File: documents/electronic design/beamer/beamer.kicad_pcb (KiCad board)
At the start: 2 copper layers, 23 parts, among them P1 CONN_01X20, P2 CONN_01X20, T1 2N7002K, T10 2N7002K, T2 2N7002K, T3 2N7002K, T4 2N7002K, T5 2N7002K, T6 2N7002K, T7 2N7002K, T8 2N7002K, T9 2N7002K, U1 NRF24L01-BRKOUT

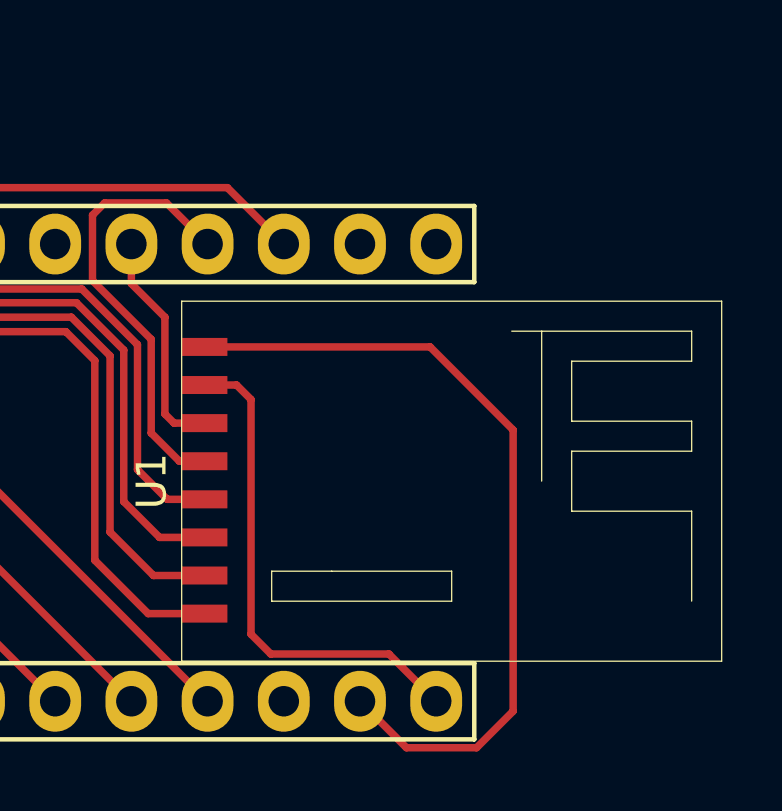
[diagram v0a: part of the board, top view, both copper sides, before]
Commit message: add capacitor to pcb
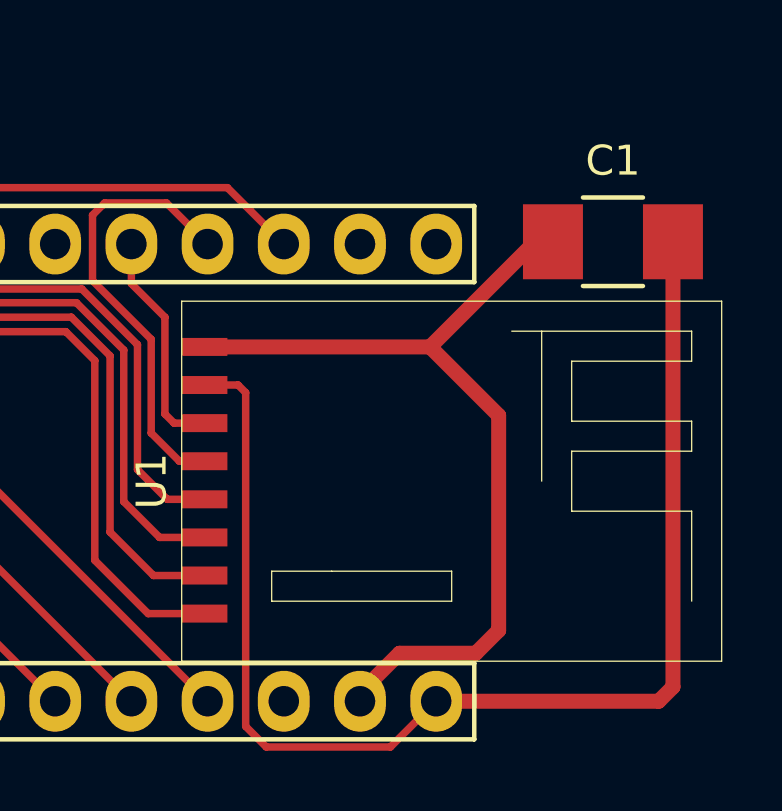
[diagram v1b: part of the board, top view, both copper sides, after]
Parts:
- added C1: C, Capacitors_SMD:C_1210_HandSoldering, F.Cu at (237.5, 44.2)
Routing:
- net +3V3: track 27.1 -> 61.3 mm
- net GND: track 30.6 -> 48.9 mm
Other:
- net class Default: trace_width 0.25 -> 0.5
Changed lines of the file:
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@@
 (kicad_pcb (version 4) (host pcbnew 4.0.2-stable)
   (general
-    (links 50)
+    (links 52)
     (no_connects 8)
-    (area 15.8222 13.9172 278.230001 189.330001)
+    (area 14.6792 16.7112 276.960001 190.3522)
     (thickness 1.6)
     (drawings 0)
-    (tracks 182)
+    (tracks 196)
     (zones 0)
-    (modules 23)
+    (modules 24)
     (nets 49)
   )
@@
     (35 F.Paste user)
     (36 B.SilkS user)
-    (37 F.SilkS user hide)
+    (37 F.SilkS user)
     (38 B.Mask user)
     (39 F.Mask user)
@@
   )
   (setup
-    (last_trace_width 0.25)
+    (last_trace_width 0.5)
     (trace_clearance 0.2)
     (zone_clearance 0.508)
@@
   (net_class Default "This is the default net class."
     (clearance 0.2)
-    (trace_width 0.25)
+    (trace_width 0.5)
     (via_dia 0.6)
     (via_drill 0.4)
@@
     (pad 3 smd rect (at 0.00254 -1.64338) (size 1 1.4) (layers F.Cu F.Paste F.Mask)
       (net 10 "Net-(D9-Pad1)") (solder_mask_margin 0.2))
+  )
+  (module Capacitors_SMD:C_1210_HandSoldering (layer F.Cu)
+    (at 237.49 44.196)
+    (descr "Capacitor SMD 1210, hand soldering")
+    (tags "capacitor 1210")
+    (attr smd)
+    (fp_text reference C1 (at 0 -2.7) (layer F.SilkS)
+      (effects (font (size 1 1) (thickness 0.15)))
+    )
+    (fp_text value C (at 0 2.7) (layer F.Fab)
+      (effects (font (size 1 1) (thickness 0.15)))
+    )
+    (fp_line (start -3.3 -1.6) (end 3.3 -1.6) (layer F.CrtYd) (width 0.05))
+    (fp_line (start -3.3 1.6) (end 3.3 1.6) (layer F.CrtYd) (width 0.05))
+    (fp_line (start -3.3 -1.6) (end -3.3 1.6) (layer F.CrtYd) (width 0.05))
+    (fp_line (start 3.3 -1.6) (end 3.3 1.6) (layer F.CrtYd) (width 0.05))
+    (fp_line (start 1 -1.475) (end -1 -1.475) (layer F.SilkS) (width 0.15))
+    (fp_line (start -1 1.475) (end 1 1.475) (layer F.SilkS) (width 0.15))
+    (pad 1 smd rect (at -2 0) (size 2 2.5) (layers F.Cu F.Paste F.Mask)
+      (net 26 GND))
+    (pad 2 smd rect (at 2 0) (size 2 2.5) (layers F.Cu F.Paste F.Mask)
+      (net 27 +3V3))
+    (model Capacitors_SMD.3dshapes/C_1210_HandSoldering.wrl
+      (at (xyz 0 0 0))
+      (scale (xyz 1 1 1))
+      (rotate (xyz 0 0 0))
+    )
   )
   (segment (start 75.1638 46.9652) (end 77.4948 46.9652) (width 0.25) (layer F.Cu) (net 1))
@@
   (segment (start 186.012 49.21) (end 213.675 49.21) (width 0.25) (layer F.Cu) (net 24))
   (segment (start 213.675 49.21) (end 223.9772 59.5122) (width 0.25) (layer F.Cu) (net 24))
+  (segment (start 235.49 44.196) (end 234.8992 44.196) (width 0.5) (layer F.Cu) (net 26))
+  (segment (start 234.8992 44.196) (end 231.394 47.7012) (width 0.5) (layer F.Cu) (net 26))
+  (segment (start 223.8756 47.7012) (end 231.394 47.7012) (width 0.5) (layer F.Cu) (net 26))
+  (segment (start 231.394 47.7012) (end 233.68 49.9872) (width 0.5) (layer F.Cu) (net 26))
+  (segment (start 233.68 49.9872) (end 233.68 57.15) (width 0.5) (layer F.Cu) (net 26))
+  (segment (start 233.68 57.15) (end 232.918 57.912) (width 0.5) (layer F.Cu) (net 26))
+  (segment (start 232.918 57.912) (end 230.378 57.912) (width 0.5) (layer F.Cu) (net 26))
+  (segment (start 230.378 57.912) (end 229.0572 59.2328) (width 0.5) (layer F.Cu) (net 26))
+  (segment (start 229.0572 59.2328) (end 229.0572 59.5122) (width 0.5) (layer F.Cu) (net 26))
+  (segment (start 229.0572 59.5122) (end 229.0572 59.2328) (width 0.25) (layer F.Cu) (net 26))
+  (segment (start 229.0572 59.2328) (end 230.378 57.912) (width 0.25) (layer F.Cu) (net 26))
+  (segment (start 230.378 57.912) (end 232.918 57.912) (width 0.25) (layer F.Cu) (net 26))
+  (segment (start 232.918 57.912) (end 233.68 57.15) (width 0.25) (layer F.Cu) (net 26))
+  (segment (start 233.68 57.15) (end 233.68 49.9872) (width 0.25) (layer F.Cu) (net 26))
+  (segment (start 233.68 49.9872) (end 231.394 47.7012) (width 0.25) (layer F.Cu) (net 26))
   (segment (start 186.012 47.31) (end 186.012 44.407) (width 0.25) (layer F.Cu) (net 26))
   (segment (start 186.012 44.407) (end 185.8772 44.2722) (width 0.25) (layer F.Cu) (net 26))
   (segment (start 183.0148 44.5946) (end 183.3372 44.2722) (width 0.25) (layer F.Cu) (net 26))
-  (segment (start 223.8756 47.7012) (end 231.394 47.7012) (width 0.25) (layer F.Cu) (net 26))
-  (segment (start 230.6066 61.0616) (end 229.0572 59.5122) (width 0.25) (layer F.Cu) (net 26))
-  (segment (start 232.9434 61.0616) (end 230.6066 61.0616) (width 0.25) (layer F.Cu) (net 26))
-  (segment (start 234.1626 59.8424) (end 232.9434 61.0616) (width 0.25) (layer F.Cu) (net 26))
-  (segment (start 234.1626 50.4698) (end 234.1626 59.8424) (width 0.25) (layer F.Cu) (net 26))
-  (segment (start 231.394 47.7012) (end 234.1626 50.4698) (width 0.25) (layer F.Cu) (net 26))
+  (segment (start 239.49 44.196) (end 239.49 59.0362) (width 0.5) (layer F.Cu) (net 27))
+  (segment (start 239.49 59.0362) (end 239.014 59.5122) (width 0.5) (layer F.Cu) (net 27))
+  (segment (start 239.014 59.5122) (end 231.5972 59.5122) (width 0.5) (layer F.Cu) (net 27))
+  (segment (start 239.014 59.5122) (end 231.5972 59.5122) (width 0.25) (layer F.Cu) (net 27))
+  (segment (start 239.49 59.0362) (end 239.014 59.5122) (width 0.25) (layer F.Cu) (net 27))
+  (segment (start 223.8756 48.9712) (end 224.9932 48.9712) (width 0.25) (layer F.Cu) (net 27))
+  (segment (start 230.0732 61.0362) (end 231.5972 59.5122) (width 0.25) (layer F.Cu) (net 27))
+  (segment (start 225.933 61.0362) (end 230.0732 61.0362) (width 0.25) (layer F.Cu) (net 27))
+  (segment (start 225.2472 60.3504) (end 225.933 61.0362) (width 0.25) (layer F.Cu) (net 27))
+  (segment (start 225.2472 49.2252) (end 225.2472 60.3504) (width 0.25) (layer F.Cu) (net 27))
+  (segment (start 224.9932 48.9712) (end 225.2472 49.2252) (width 0.25) (layer F.Cu) (net 27))
   (segment (start 179.832 43.862) (end 180.166 43.862) (width 0.25) (layer F.Cu) (net 27))
   (segment (start 180.166 43.862) (end 181.356 42.672) (width 0.25) (layer F.Cu) (net 27))
   (segment (start 181.356 42.672) (end 186.817 42.672) (width 0.25) (layer F.Cu) (net 27))
   (segment (start 186.817 42.672) (end 188.4172 44.2722) (width 0.25) (layer F.Cu) (net 27))
-  (segment (start 223.8756 48.9712) (end 224.9424 48.9712) (width 0.25) (layer F.Cu) (net 27))
-  (segment (start 230.0224 57.9374) (end 231.5972 59.5122) (width 0.25) (layer F.Cu) (net 27))
-  (segment (start 226.0854 57.9374) (end 230.0224 57.9374) (width 0.25) (layer F.Cu) (net 27))
-  (segment (start 225.425 57.277) (end 226.0854 57.9374) (width 0.25) (layer F.Cu) (net 27))
-  (segment (start 225.425 49.4538) (end 225.425 57.277) (width 0.25) (layer F.Cu) (net 27))
-  (segment (start 224.9424 48.9712) (end 225.425 49.4538) (width 0.25) (layer F.Cu) (net 27))
   (segment (start 223.8756 48.9712) (end 224.536 48.9712) (width 0.25) (layer F.Cu) (net 27))
+  (segment (start 95.25 56.134) (end 200.279 56.134) (width 0.25) (layer F.Cu) (net 31))
+  (segment (start 91.7358 52.6198) (end 95.25 56.134) (width 0.25) (layer F.Cu) (net 31))
   (segment (start 91.7358 49.41834) (end 91.7358 52.6198) (width 0.25) (layer F.Cu) (net 31))
   (segment (start 200.279 56.134) (end 203.6572 59.5122) (width 0.25) (layer F.Cu) (net 31))
-  (segment (start 95.25 56.134) (end 200.279 56.134) (width 0.25) (layer F.Cu) (net 31))
-  (segment (start 91.7358 52.6198) (end 95.25 56.134) (width 0.25) (layer F.Cu) (net 31))
   (segment (start 79.7358 49.41834) (end 79.7358 52.0498) (width 0.25) (layer F.Cu) (net 32))
   (segment (start 198.501 56.896) (end 201.1172 59.5122) (width 0.25) (layer F.Cu) (net 32))
